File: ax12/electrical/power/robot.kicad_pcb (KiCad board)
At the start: 2 copper layers, 49.5 x 49.5 mm, 33 parts, among them J1 LEG1, J2 LEG2, J3 LEG4, J4 LEG3, J5 Data P, J6 PWR IN, U1 LM317_12, U2 LM317_12, U3 LM317_34, U4 LM317_34

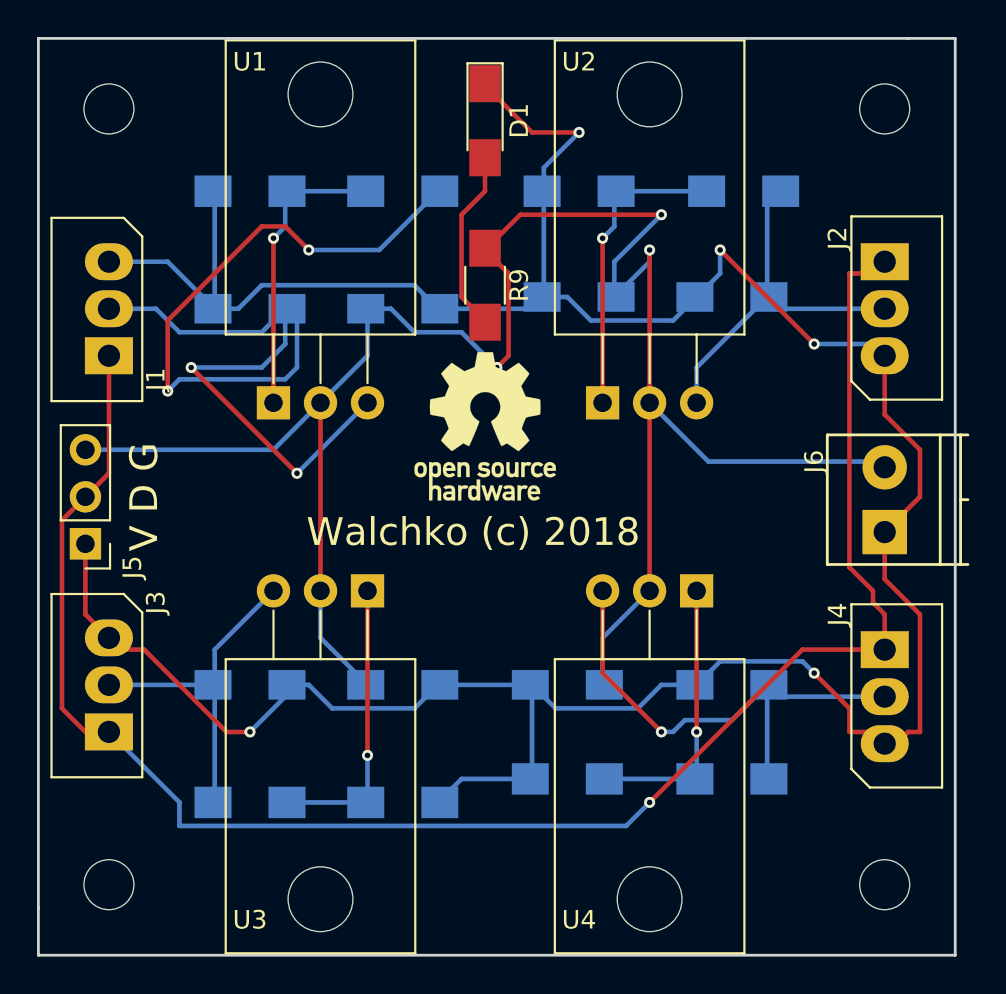
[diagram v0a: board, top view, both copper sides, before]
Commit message: updates
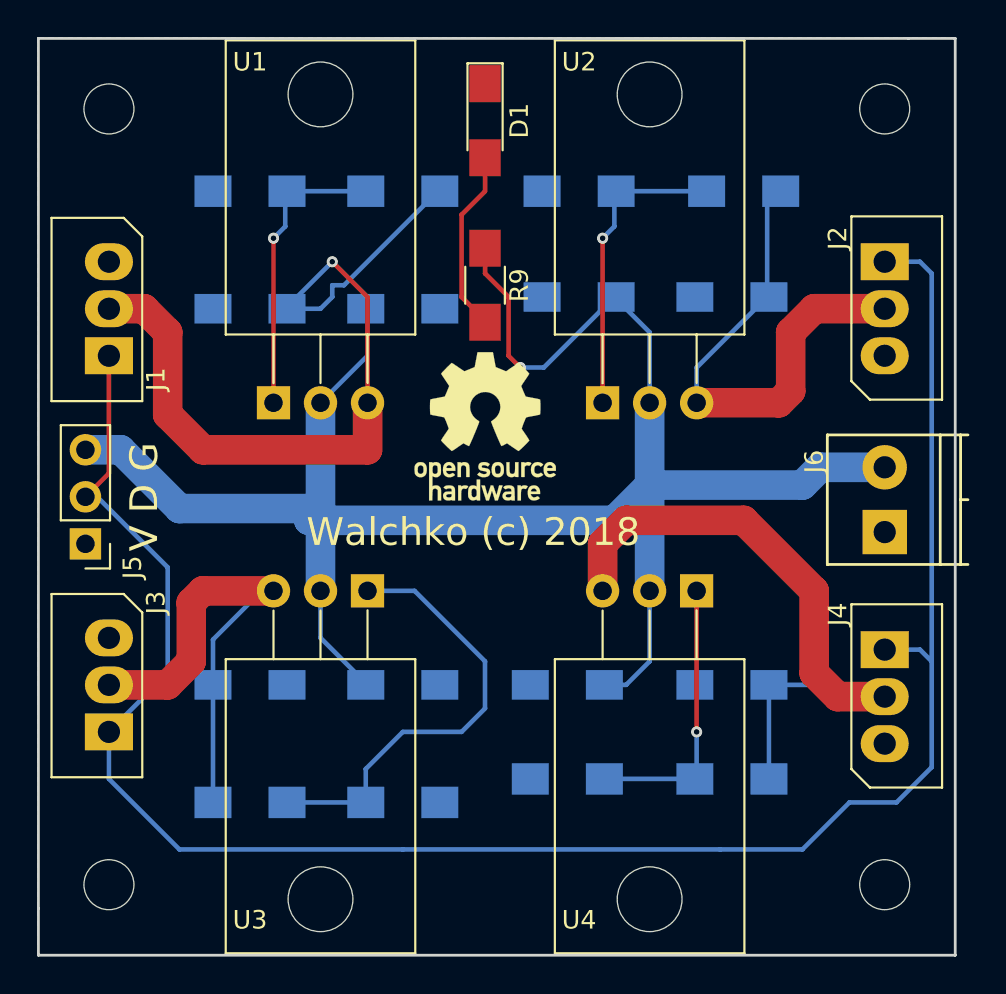
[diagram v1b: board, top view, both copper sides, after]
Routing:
- net GNDA: track 164.8 -> 0.00 mm, vias 5 -> 0
- net Net-(C3-Pad1): track 65.2 -> 45.6 mm, vias 4 -> 1
- net DATA: track 95.1 -> 107.1 mm, vias 1 -> 0
- net Net-(C6-Pad1): track 27.8 -> 36.5 mm, vias 1 -> 0
- net Net-(R5-Pad2): track 15.8 -> 24.3 mm, vias 1 -> 0
- net Net-(C4-Pad1): track 20.3 -> 27.7 mm
- net Net-(C5-Pad1): track 18.7 -> 26.0 mm
- net +VDC: track 110.4 -> 107.2 mm, vias 3 -> 1
- added copper zone on B.Cu, net GNDA
- added copper zone on F.Cu, net GNDA
